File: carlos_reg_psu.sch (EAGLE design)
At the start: 13 parts

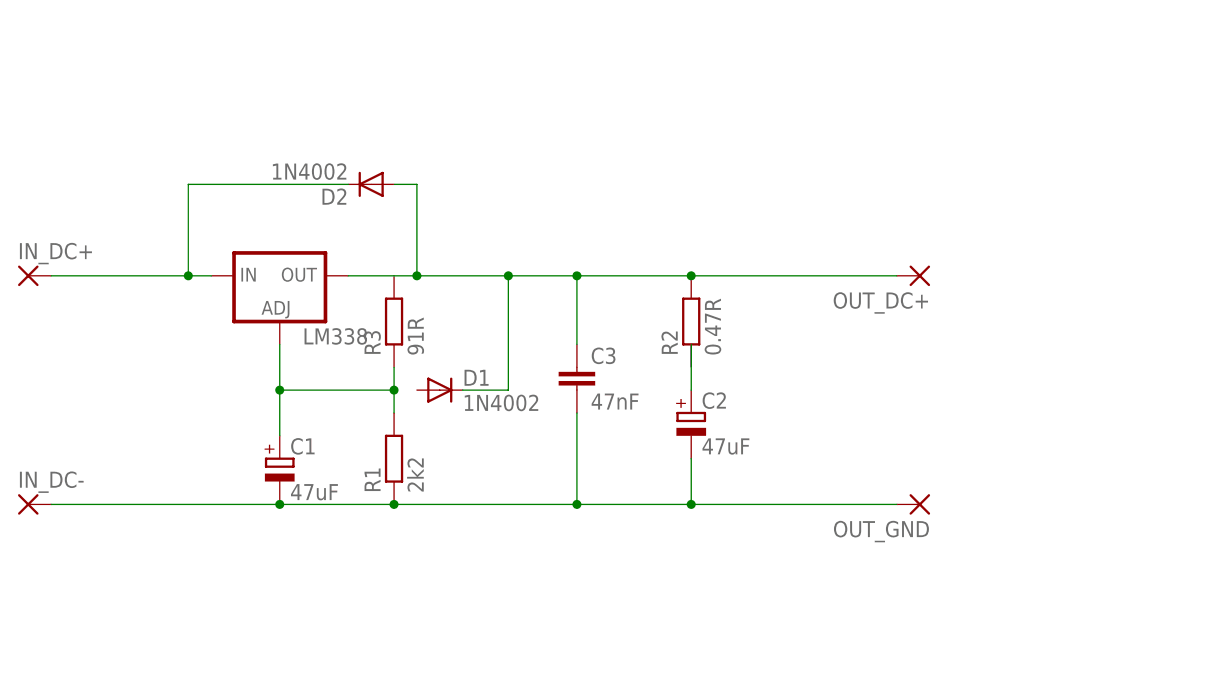
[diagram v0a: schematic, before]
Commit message: rev0 finished
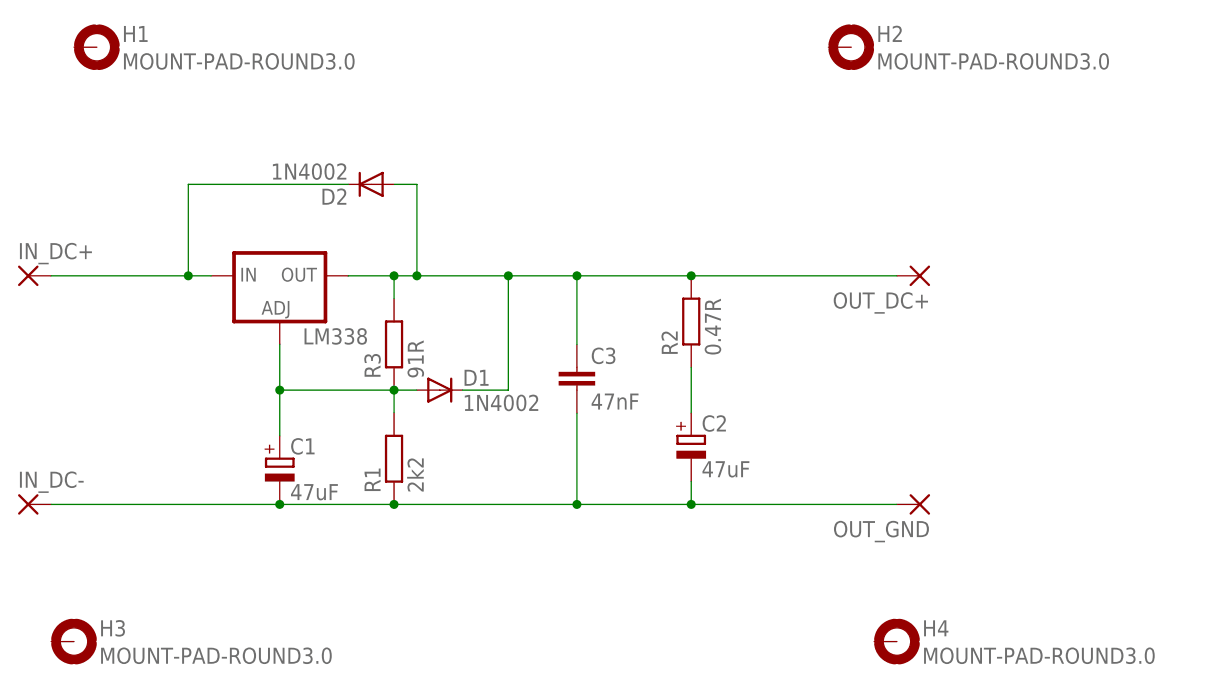
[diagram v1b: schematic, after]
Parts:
- added H1, H2, H3, H4: MOUNT-PAD-ROUND3.0, holes:MOUNT-PAD-ROUND3.0
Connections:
- removed net N$5: C2.+
- new net N$1: C2.+, R2.1
- net N$2: now also D1.A
- net N$3: now also R3.2
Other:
- moved on the sheet: C2, R3
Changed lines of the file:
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@@
 <part name="OUT_DC+" library="wirepad" deviceset="2,54/1,0" device=""/>
 <part name="OUT_GND" library="wirepad" deviceset="2,54/1,0" device=""/>
+<part name="H1" library="holes" deviceset="MOUNT-PAD-ROUND" device="3.0"/>
+<part name="H2" library="holes" deviceset="MOUNT-PAD-ROUND" device="3.0"/>
+<part name="H3" library="holes" deviceset="MOUNT-PAD-ROUND" device="3.0"/>
+<part name="H4" library="holes" deviceset="MOUNT-PAD-ROUND" device="3.0"/>
 </parts>
 <sheets>
@@
 <instance part="D2" gate="1" x="73.66" y="60.96" rot="R180"/>
 <instance part="C1" gate="G$1" x="63.5" y="30.48"/>
-<instance part="C2" gate="G$1" x="109.22" y="35.56"/>
+<instance part="C2" gate="G$1" x="109.22" y="33.02"/>
 <instance part="R1" gate="G$1" x="76.2" y="30.48" rot="R90"/>
 <instance part="R2" gate="G$1" x="109.22" y="45.72" rot="R90"/>
-<instance part="R3" gate="G$1" x="76.2" y="45.72" rot="R90"/>
+<instance part="R3" gate="G$1" x="76.2" y="43.18" rot="R90"/>
 <instance part="C3" gate="G$1" x="96.52" y="40.64"/>
 <instance part="IN_DC+" gate="P" x="35.56" y="50.8"/>
@@
 <instance part="OUT_DC+" gate="P" x="134.62" y="50.8" rot="R180"/>
 <instance part="OUT_GND" gate="P" x="134.62" y="25.4" rot="R180"/>
+<instance part="H1" gate="G$1" x="43.18" y="76.2"/>
+<instance part="H2" gate="G$1" x="127" y="76.2"/>
+<instance part="H3" gate="G$1" x="40.64" y="10.16"/>
+<instance part="H4" gate="G$1" x="132.08" y="10.16"/>
 </instances>
 <busses>
@@
 <pinref part="R3" gate="G$1" pin="1"/>
 <pinref part="R1" gate="G$1" pin="2"/>
-<wire x1="76.2" y1="40.64" x2="76.2" y2="38.1" width="0.1524" layer="91"/>
 <pinref part="LM338" gate="1" pin="ADJ"/>
 <pinref part="C1" gate="G$1" pin="+"/>
@@
 <junction x="76.2" y="38.1"/>
 <junction x="63.5" y="38.1"/>
+<pinref part="D1" gate="1" pin="A"/>
+<wire x1="76.2" y1="38.1" x2="78.74" y2="38.1" width="0.1524" layer="91"/>
 </segment>
 </net>
@@
 <segment>
 <pinref part="LM338" gate="1" pin="OUT"/>
-<wire x1="71.12" y1="50.8" x2="78.74" y2="50.8" width="0.1524" layer="91"/>
+<wire x1="71.12" y1="50.8" x2="76.2" y2="50.8" width="0.1524" layer="91"/>
+<wire x1="76.2" y1="50.8" x2="78.74" y2="50.8" width="0.1524" layer="91"/>
 <wire x1="78.74" y1="50.8" x2="88.9" y2="50.8" width="0.1524" layer="91"/>
 <wire x1="88.9" y1="50.8" x2="88.9" y2="38.1" width="0.1524" layer="91"/>
@@
 <wire x1="109.22" y1="50.8" x2="132.08" y2="50.8" width="0.1524" layer="91"/>
 <junction x="109.22" y="50.8"/>
+<pinref part="R3" gate="G$1" pin="2"/>
+<wire x1="76.2" y1="50.8" x2="76.2" y2="48.26" width="0.1524" layer="91"/>
+<junction x="76.2" y="50.8"/>
 </segment>
 </net>
@@
 </segment>
 </net>
-<net name="N$5" class="0">
-<segment>
-<pinref part="C2" gate="G$1" pin="+"/>
-<wire x1="109.22" y1="43.18" x2="109.22" y2="38.1" width="0.1524" layer="91"/>
-</segment>
-</net>
 <net name="N$6" class="0">
 <segment>
@@
 <wire x1="76.2" y1="25.4" x2="96.52" y2="25.4" width="0.1524" layer="91"/>
 <wire x1="96.52" y1="25.4" x2="109.22" y2="25.4" width="0.1524" layer="91"/>
-<wire x1="109.22" y1="25.4" x2="109.22" y2="30.48" width="0.1524" layer="91"/>
+<wire x1="109.22" y1="25.4" x2="109.22" y2="27.94" width="0.1524" layer="91"/>
 <junction x="76.2" y="25.4"/>
 <pinref part="C3" gate="G$1" pin="2"/>
@@
 </segment>
 </net>
+<net name="N$1" class="0">
+<segment>
+<pinref part="C2" gate="G$1" pin="+"/>
+<pinref part="R2" gate="G$1" pin="1"/>
+<wire x1="109.22" y1="35.56" x2="109.22" y2="40.64" width="0.1524" layer="91"/>
+</segment>
+</net>
